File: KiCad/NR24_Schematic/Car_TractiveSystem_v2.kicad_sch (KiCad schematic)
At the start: 15 parts, among them J1 M_con, J2 F_con, K2 Key Switch Relay, M1 Zero_7R_Motor, SW3 100V E-stop (Right), SW4 100V E-stop (Left), SW7 TI power switch, SW8 GLVMS, U1 Sevcon_Gen4_Size6, U2 Throttle, U7 Brake (AiM Pressure Sensor)

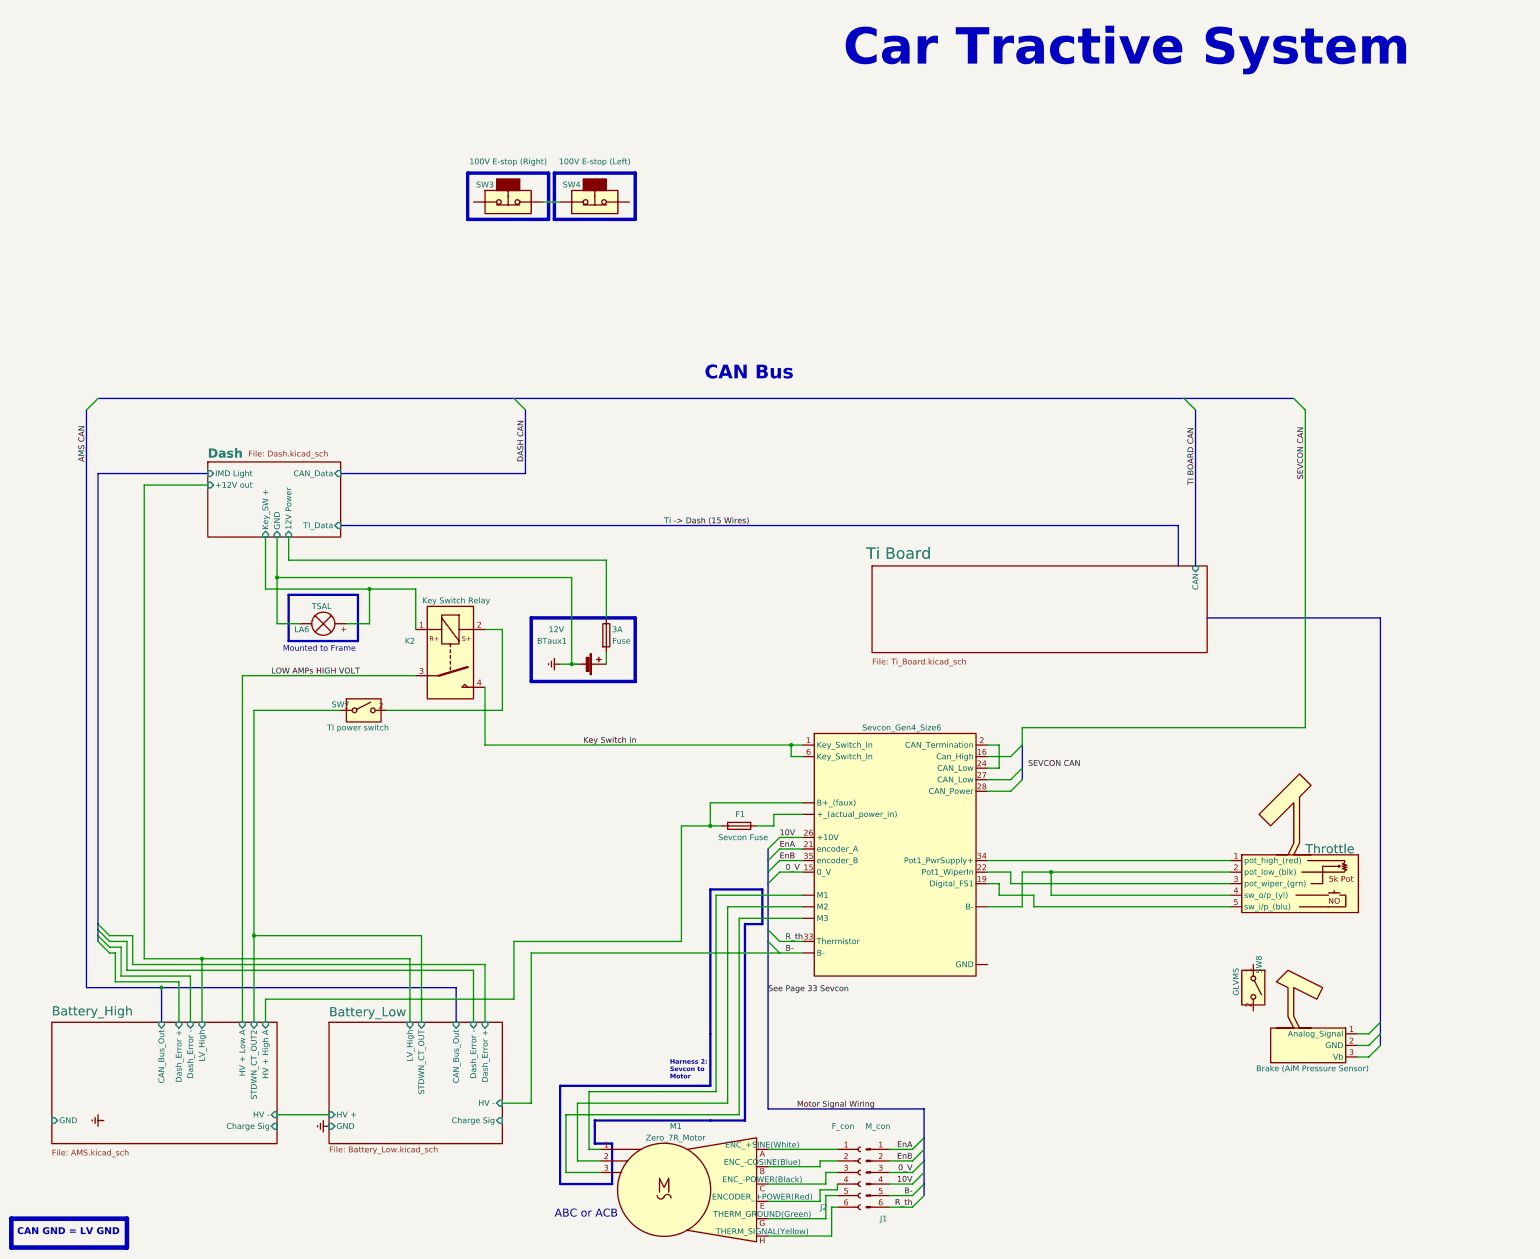
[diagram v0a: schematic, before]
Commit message: .
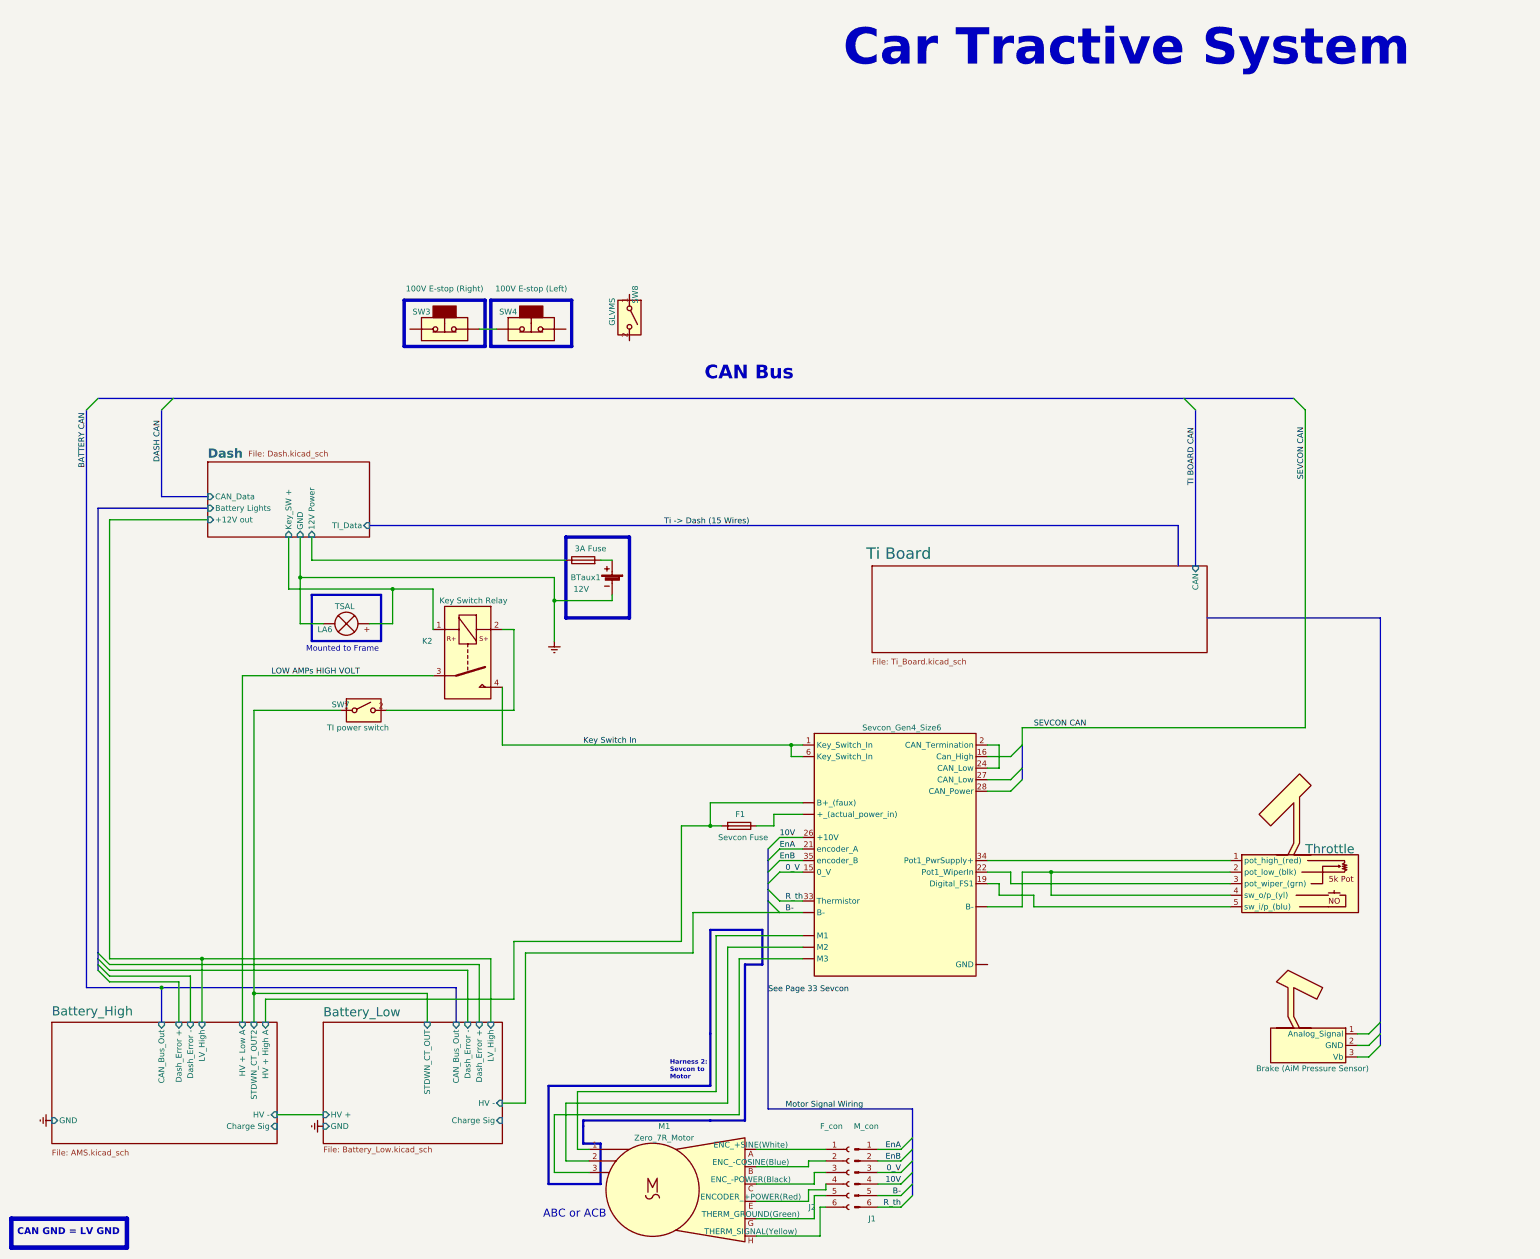
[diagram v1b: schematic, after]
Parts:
- 3A: value Fuse -> 3A Fuse
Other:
- sheet Dash ports: added Battery Lights; removed IMD Light
- moved on the sheet: J1, J2, K2, LA6, M1, SW3, SW4, SW8

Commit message: Now it is pretty :)
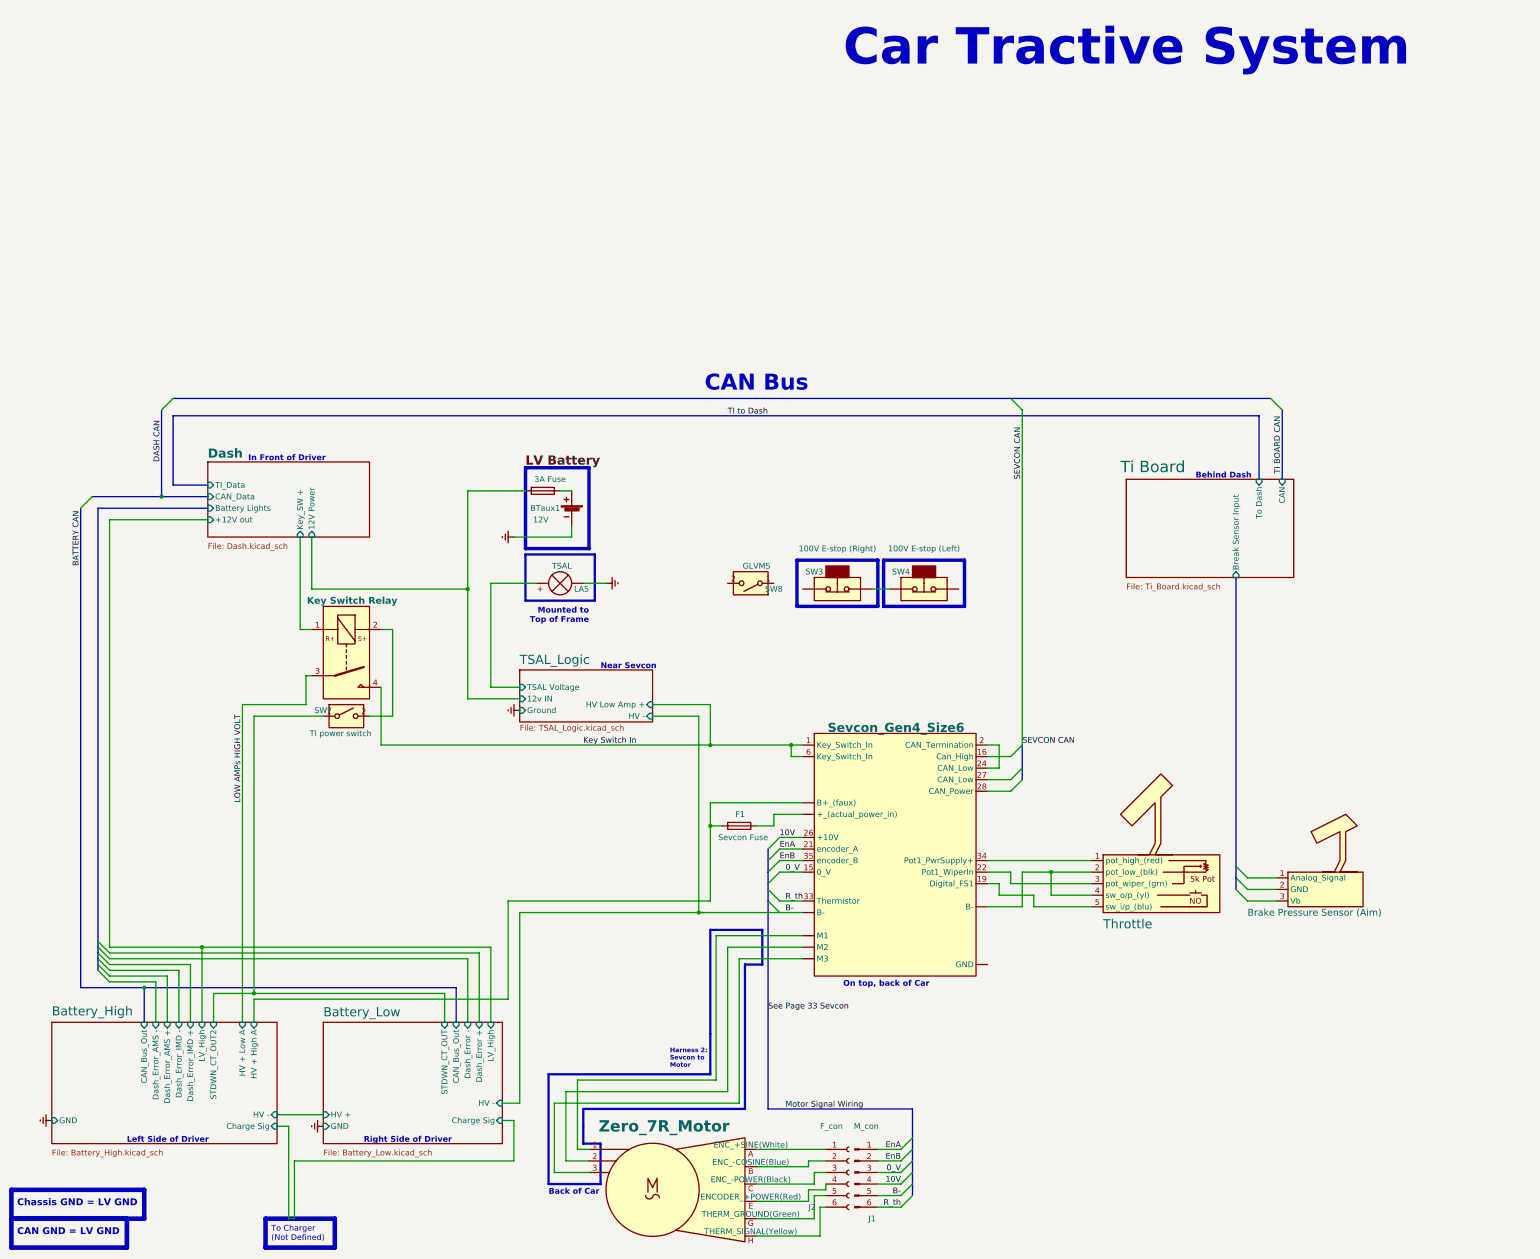
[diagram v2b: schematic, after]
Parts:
- removed LA6: TSAL, symbol Device:Lamp
- added LA5: TSAL, symbol Device:Lamp
- U7: value Brake (AiM Pressure Sensor) -> Brake Pressure Sensor (Aim)
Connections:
- net Earth: now also LA5.1 (-)
- new net TSAL_Logic/TSAL Voltage: LA5.2 (+)
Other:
- added sheet TSAL_Logic (TSAL_Logic.kicad_sch)
- sheet Battery_High: file AMS.kicad_sch -> Battery_High.kicad_sch
- sheet Battery_High ports: added Dash_Error_AMS +, Dash_Error_AMS -, Dash_Error_IMD +, Dash_Error_IMD -; removed Dash_Error +, Dash_Error -
- sheet Dash ports: added none; removed GND
- sheet Ti Board ports: added Break Sensor Input, To Dash; removed none
- note added: "Back of Car"
- note added: "Behind Dash"
- note added: "Chassis GND = LV GND"
- note added: "In Front of Driver"
- note added: "Left Side of Driver"
- note added: "Mounted to Top of Frame"
- note added: "Near Sevcon"
- note added: "On top, back of Car"
- note added: "Right Side of Driver"
- note added: "To Charger (Not Defined)"
- note removed: "ABC or ACB"
- note removed: "Mounted to Frame"
- moved on the sheet: BTaux1, SW3, SW4, SW7, SW8
